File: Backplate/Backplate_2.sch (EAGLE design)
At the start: 13 parts, among them J1 1725672, J2 1725672, J3 1725698, J4 1725672, J6 5.5x2.1mm Barrel, Q1 QTPY

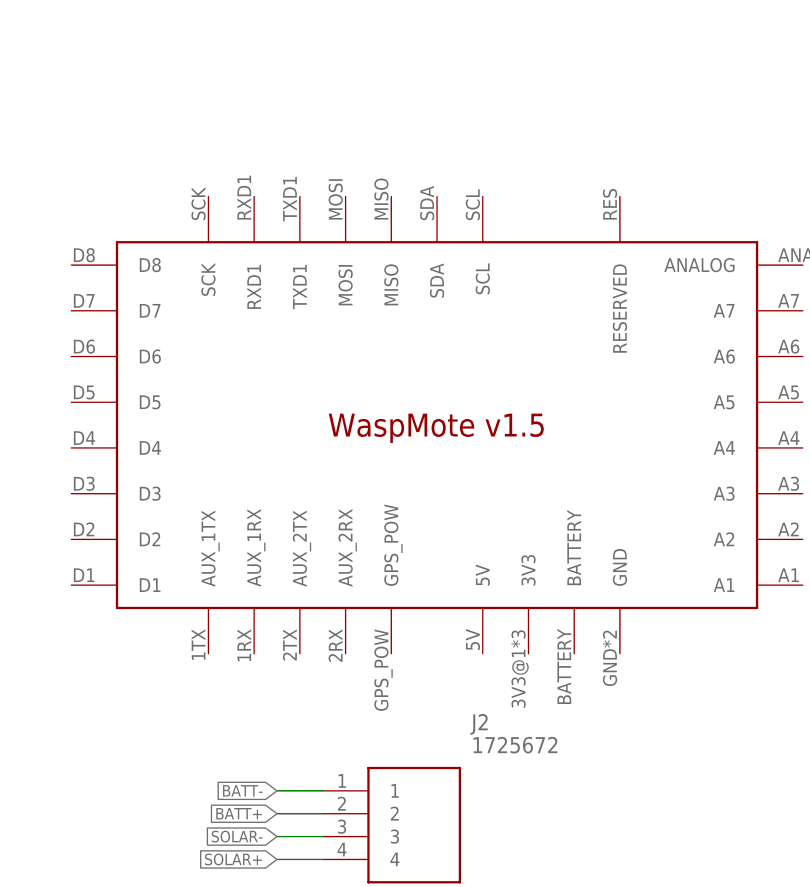
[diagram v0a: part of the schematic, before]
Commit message: Flamingo PCB
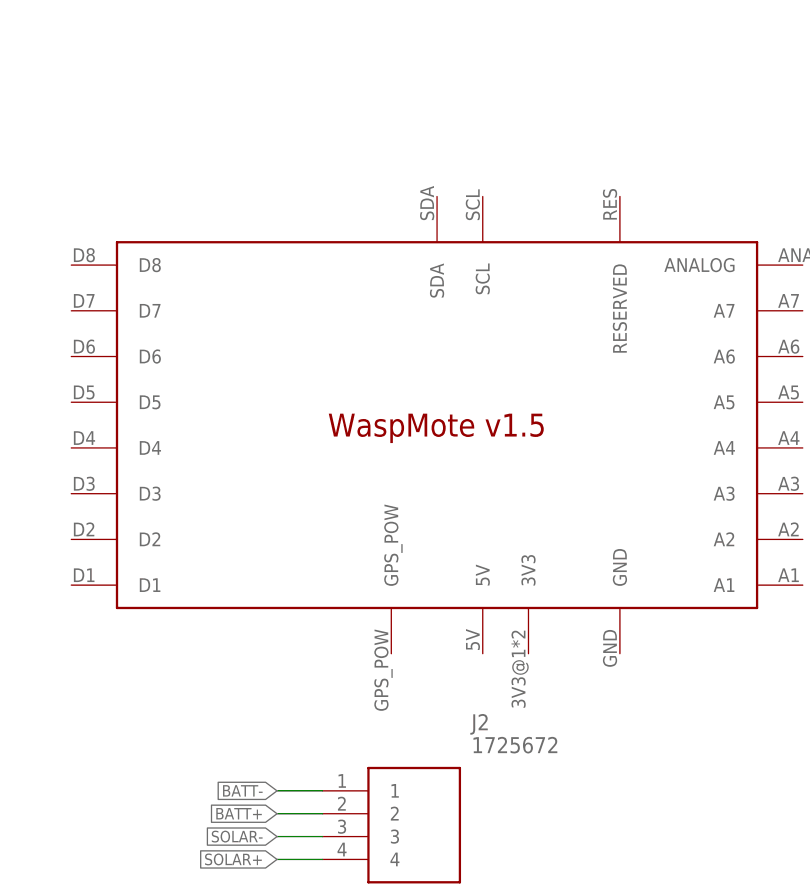
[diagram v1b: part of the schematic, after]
